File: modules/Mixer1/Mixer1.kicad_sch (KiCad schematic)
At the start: 40 parts, among them U1 TL074, U2 TL074, U3 TL072

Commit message: Mixer1 - wip
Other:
- title: Eurorack Dual Mixer -> Eurorack Mixer
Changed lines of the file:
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@@
   (paper "A4")
   (title_block
-    (title "Eurorack Dual Mixer")
-    (date "2022-10-03")
-    (rev "1.2")
+    (title "Eurorack Mixer")
+    (date "2022-11-13")
+    (rev "1.0")
     (company "Len Popp")
     (comment 1 "Copyright © 2022 Len Popp CC BY")
-    (comment 2 "Layout designed for 8HP module using Delptronics Module Construction Set")
-    (comment 3 "Eurorack 2-channel 3:1 mixer module - 8HP")
+    (comment 2 "Eurorack 3:1 mixer module - 4HP")
   )
   (junction (at 77.47 107.95) (diameter 0) (color 0 0 0 0)

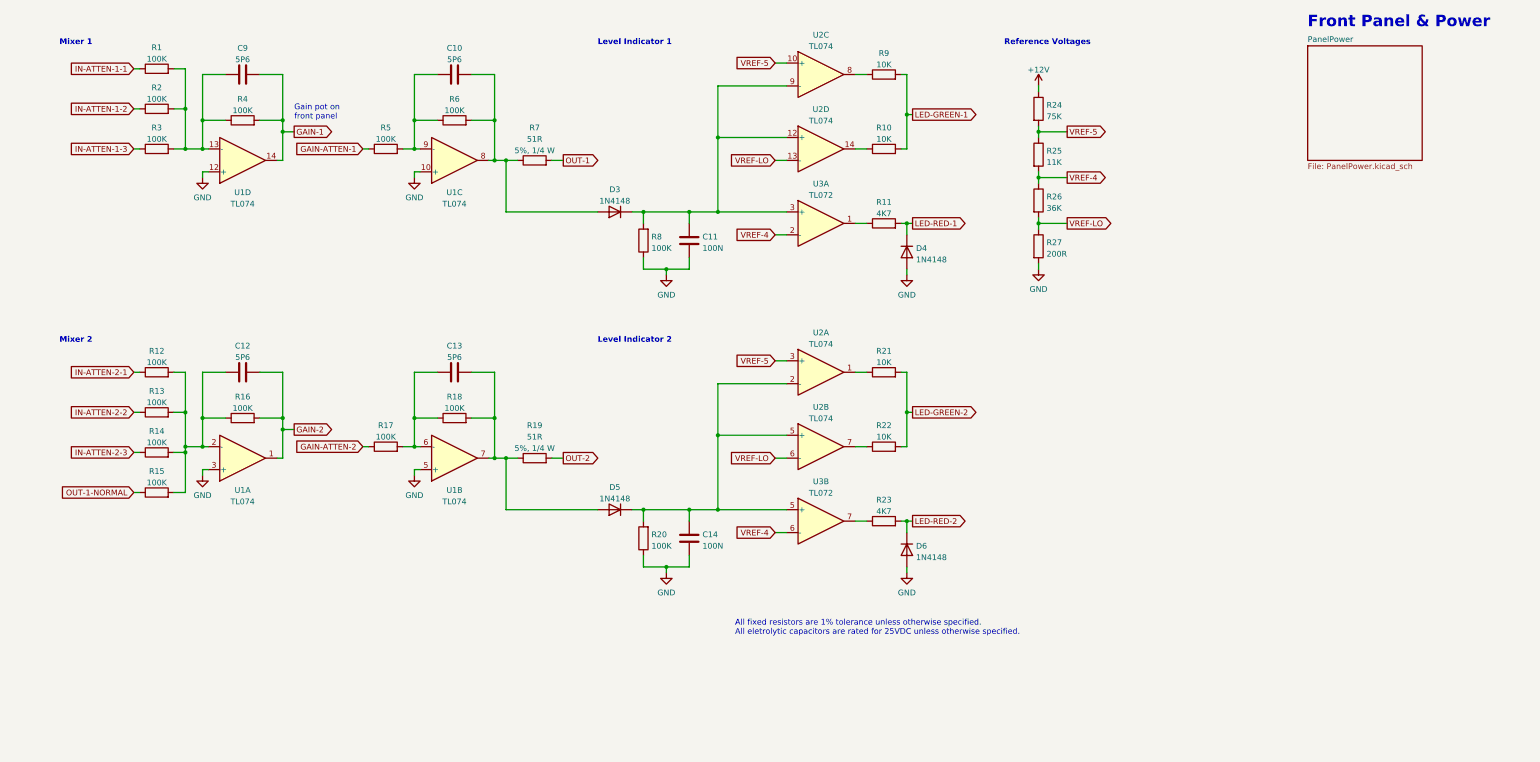
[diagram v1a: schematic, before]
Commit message: Mixer1 - wip
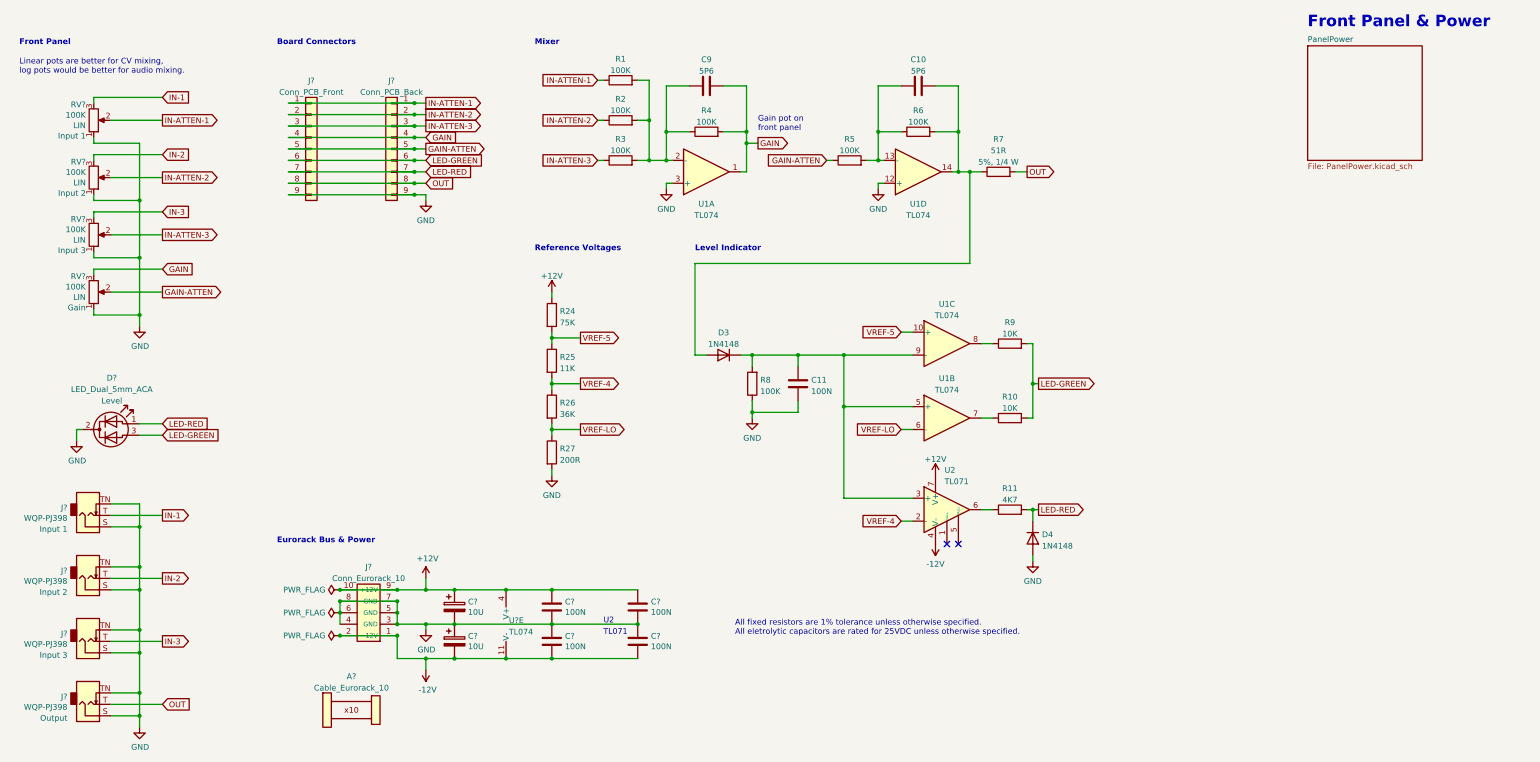
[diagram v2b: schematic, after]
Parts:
- removed C12, C13: 5P6, -lmp-misc:C_Disc_D5.0mm_W2.5mm_P2.50mm, symbol -lmp:CC
- removed C14: 100N, -lmp-misc:C_Disc_D5.0mm_W2.5mm_P2.50mm, symbol -lmp:CC_100N
- removed D5, D6: 1N4148, Diode_THT:D_DO-35_SOD27_P7.62mm_Horizontal, symbol -lmp-diode:1N4148
- removed R12, R13, R14, R15, R16, R17, R18, R20: 100K, -lmp-misc:R_Axial_DIN0207_L6.3mm_D2.5mm_P7.62mm_Horizontal, symbol -lmp:R_1%_0W166
- removed R19: 51R, -lmp-misc:R_Axial_DIN0207_L6.3mm_D2.5mm_P10.16mm_Horizontal, symbol -lmp-synth:R_51R_Output
- removed R21, R22: 10K, -lmp-misc:R_Axial_DIN0207_L6.3mm_D2.5mm_P7.62mm_Horizontal, symbol -lmp:R_1%_0W166
- removed R23: 4K7, -lmp-misc:R_Axial_DIN0207_L6.3mm_D2.5mm_P7.62mm_Horizontal, symbol -lmp:R_1%_0W166
- removed unit 2 of U1
- removed unit 1 of U1
- removed unit 2 of U2
- removed unit 1 of U2
- removed U3: TL072, Package_DIP:DIP-8_W7.62mm, symbol -lmp-opamp:TL072
- added A?: Cable_Eurorack_10, -lmp-misc:NoFootprint, symbol -lmp-synth:Cable_Eurorack_10
- added C? (x4): 100N, -lmp-misc:C_Disc_D5.0mm_W2.5mm_P2.50mm, symbol -lmp:CC_100N
- added C? (x2): 10U, -lmp-misc:CP_Radial_D5.0mm_P2.50mm, symbol -lmp-synth:CP_10U
- added D?: LED_Dual_5mm_ACA, LED_THT:LED_D5.0mm-3, symbol -lmp-synth:LED_Dual_5mm_Red_Green_ACA
- added J?: Conn_PCB_Front, Connector_PinSocket_2.54mm:PinSocket_1x09_P2.54mm_Vertical, symbol Connector_Generic:Conn_01x09
- added J? (x4): WQP-PJ398, -lmp-synth:Jack_3.5mm_QingPu_WQP-PJ398SM_Vertical, symbol -lmp-synth:Jack_WQP-PJ398
- added J?: Conn_PCB_Back, Connector_PinHeader_2.54mm:PinHeader_1x09_P2.54mm_Vertical, symbol Connector_Generic:Conn_01x09
- added J?: Conn_Eurorack_10, -lmp-synth:IDC-Header-Eurorack-10-TH, symbol -lmp-synth:Conn_Eurorack_Pwr_10
- added RV? (x4): 100K, -lmp-synth:Potentiometer_Alpha_RD901F-40-00D_Single_Vertical, symbol -lmp-synth:R_POT_Panel_PCB_Alpha
- added U2: TL071, Package_DIP:DIP-8_W7.62mm, symbol -lmp-opamp:TL071
- added U?: TL074, Package_DIP:DIP-14_W7.62mm, symbol -lmp-opamp:TL074
- renumbered U2 to U1
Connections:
- net +12V: now also C?.1, C?.1, C?.1, J?.10, J?.9 (+12V), U2.7 (V+), U?.4 (V+)
- net GND: now also U1.12 (+), U1.3 (+), C?.1, C?.1, C?.1, C?.2, C?.2, C?.2, D?.2 (K), J?.3 (GND), J?.4, J?.5 (GND), J?.6, J?.7 (GND), J?.8, J?.9 (Pin_9), J?.9 (Pin_9), J?.S, J?.S, J?.S, J?.S, J?.TN, J?.TN, J?.TN, J?.TN, RV?.1, RV?.1, RV?.1, RV?.1; no longer U1.10 (+), U1.12 (+)
- net VREF-4: now also U2.2 (-)
- net VREF-LO: now also U1.6 (-); no longer U1.13 (-)
- net at C9.1, R1.2, R2.2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: now also U1.2 (-); no longer U1.13 (-)
- net at C10.1, R5.2, R6.1: now also U1.13 (-); no longer U1.9 (-)
- net at C10.2, D3.2 (A), R6.2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: now also U1.14; no longer U1.8
- net at R11.1: now also U2.6
- net at C11.1, D3.1 (K), R8.2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: now also U1.5 (+), U2.3 (+); no longer U1.12 (+)
- net at R10.1: now also U1.7; no longer U1.14
- net GAIN-1 renamed GAIN
- net GAIN: now also U1.1, J?.4 (Pin_4), J?.4 (Pin_4), RV?.3; no longer U1.14
- net GAIN-ATTEN-1 renamed GAIN-ATTEN
- net GAIN-ATTEN: now also J?.5 (Pin_5), J?.5 (Pin_5), RV?.2
- net IN-ATTEN-1-1 renamed IN-ATTEN-1
- net IN-ATTEN-1: now also J?.1 (Pin_1), J?.1 (Pin_1), RV?.2
- net IN-ATTEN-1-2 renamed IN-ATTEN-2
- net IN-ATTEN-2: now also J?.2 (Pin_2), J?.2 (Pin_2), RV?.2
- net IN-ATTEN-1-3 renamed IN-ATTEN-3
- net IN-ATTEN-3: now also J?.3 (Pin_3), J?.3 (Pin_3), RV?.2
- net LED-GREEN-1 renamed LED-GREEN
- net LED-GREEN: now also D?.3 (A2), J?.6 (Pin_6), J?.6 (Pin_6)
- net LED-RED-1 renamed LED-RED
- net LED-RED: now also D?.1 (A1), J?.7 (Pin_7), J?.7 (Pin_7)
- net OUT-1 renamed OUT
- net OUT: now also J?.8 (Pin_8), J?.8 (Pin_8), J?.T
- new net -12V: C?.2, C?.2, C?.2, J?.1 (-12V), J?.2, U2.4 (V-), U?.11 (V-)
- new net IN-1: J?.T, RV?.3
- new net IN-2: J?.T, RV?.3
- new net IN-3: J?.T, RV?.3
- no-connect marks 0 -> 2
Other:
- note added: "Board Connectors"
- note added: "Eurorack Bus & Power"
- note added: "Front Panel"
- note added: "Level Indicator"
- note added: "Linear pots are better for CV mixing, log pots would be better for audio mixing."
- note added: "Mixer"
- note added: "TL071"
- note added: "U2"
- note removed: "Level Indicator 1"
- note removed: "Level Indicator 2"
- note removed: "Mixer 1"
- note removed: "Mixer 2"
- moved on the sheet: C10, C11, C9, D3, D4, R1, R10, R11, R2, R24, R25, R26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
